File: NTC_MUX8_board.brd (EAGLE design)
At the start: 76.2 x 63.5 mm, 65 parts, among them IC1 NINA-B306-00B-00, IC2 INA126E, IC3 MCP6001T_SOT23, IC4 MAX8559ETAAA+T, J1 USB4105-GF-A, J2 1761681-7, J3 DM3CS-SF-PEJMS, J4 DNP, J7 52808-2071, U1 TMUX1208PWR, U2 TMUX1208PWR, U3 TMUX1208PWR, U4 TMUX1208PWR, X1 22-23-2021

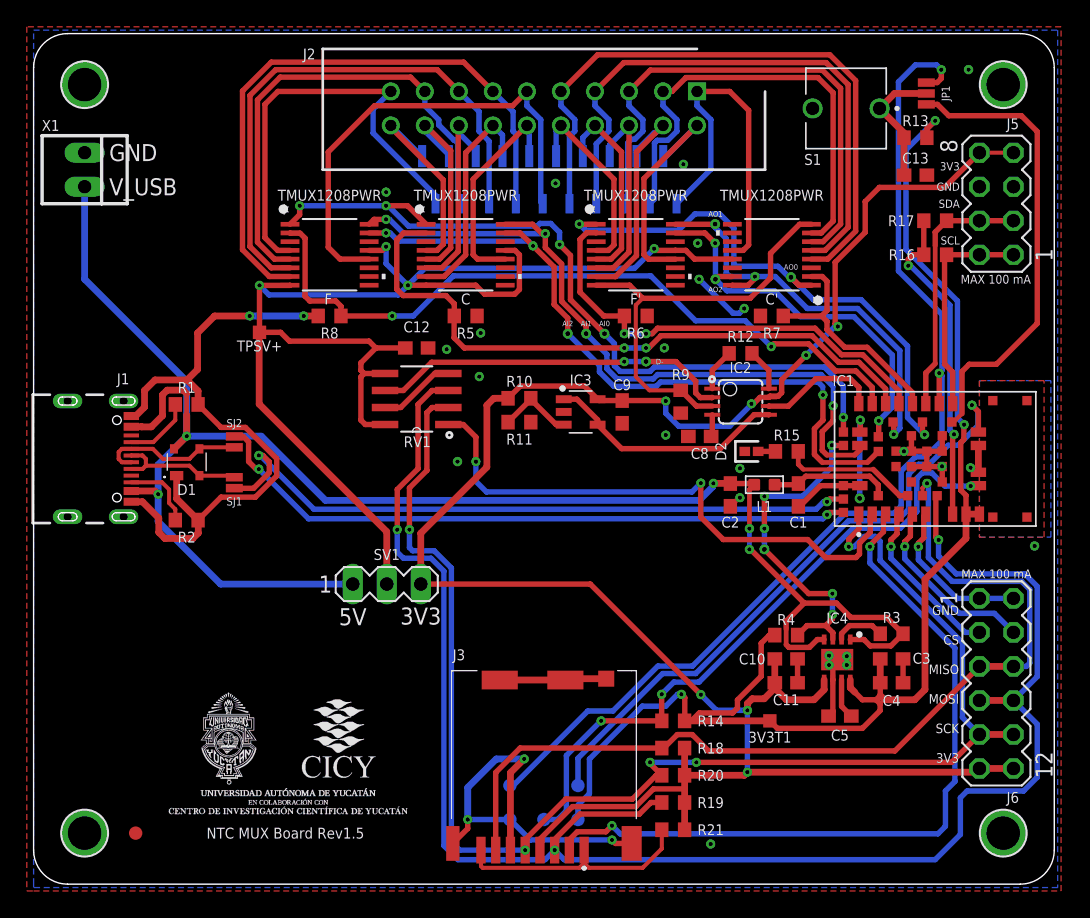
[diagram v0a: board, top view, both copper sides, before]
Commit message: beta finalizada
circuito listo a mi parecer
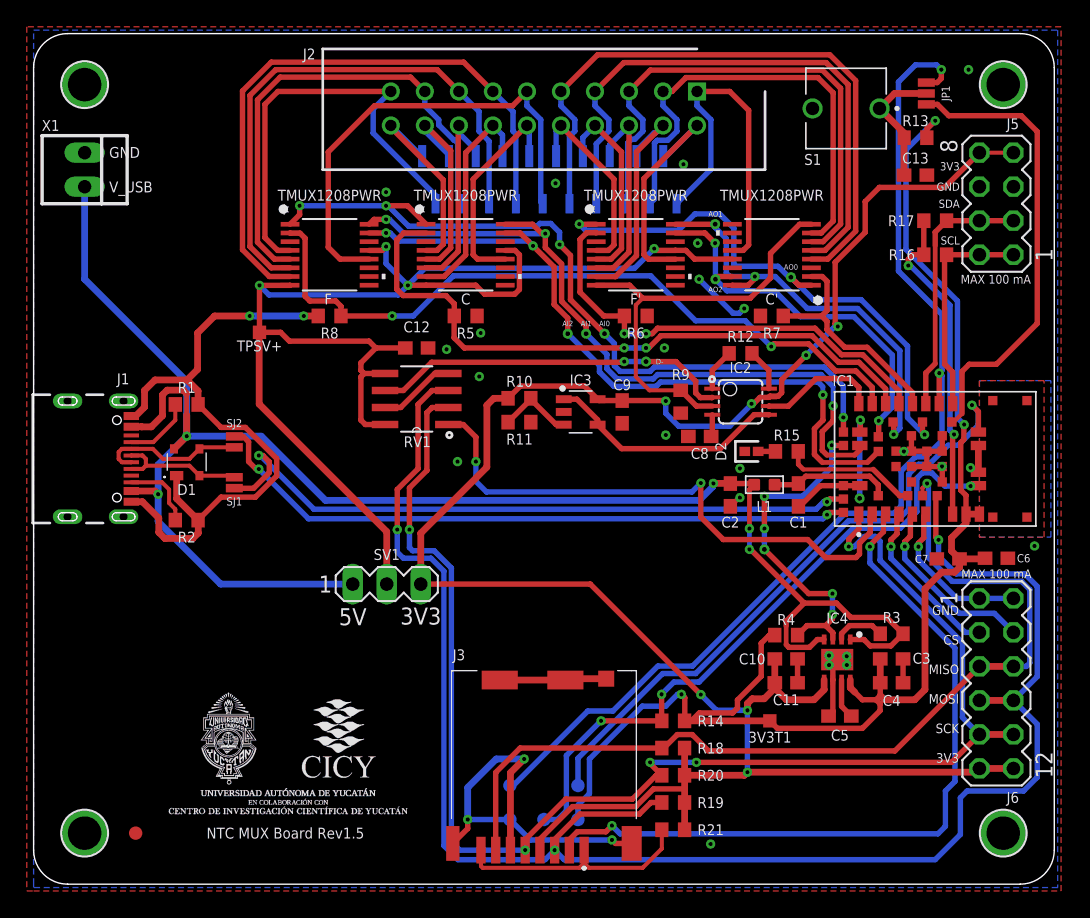
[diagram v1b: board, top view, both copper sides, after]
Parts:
- added C6, C7: 100nF, rcl:C0603
- C10, C3: value 2.2uF -> 100nF
- C11, C4: value 2.2uF -> 10uF
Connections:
- net 3V3_1: now also C6.1, C7.1
- net GND: now also C6.2, C7.2
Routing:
- net 3V3_1: track 102.4 -> 105.4 mm
